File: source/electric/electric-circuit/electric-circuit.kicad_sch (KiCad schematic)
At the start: 7 parts

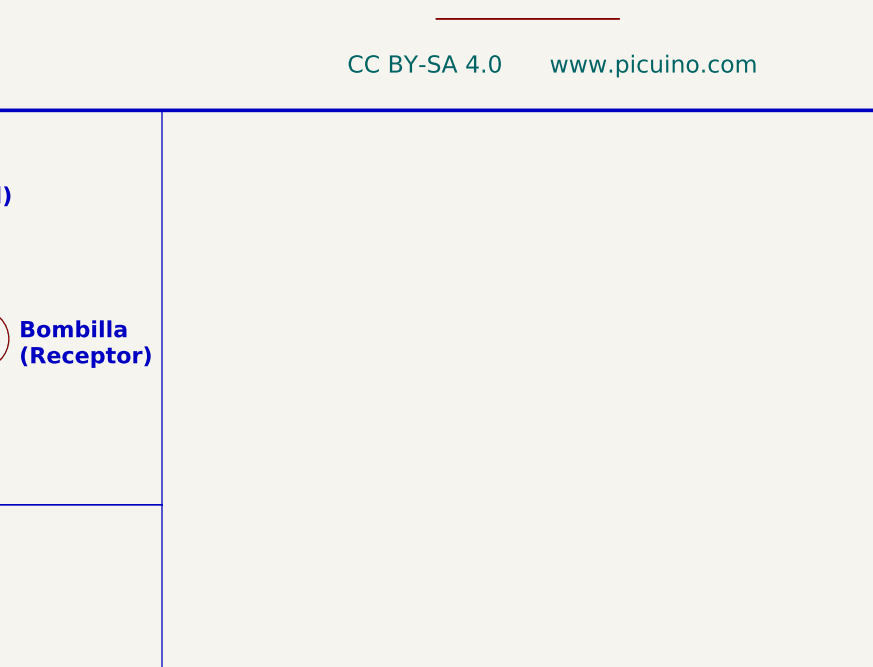
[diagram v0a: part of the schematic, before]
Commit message: 02/09/2024 Update
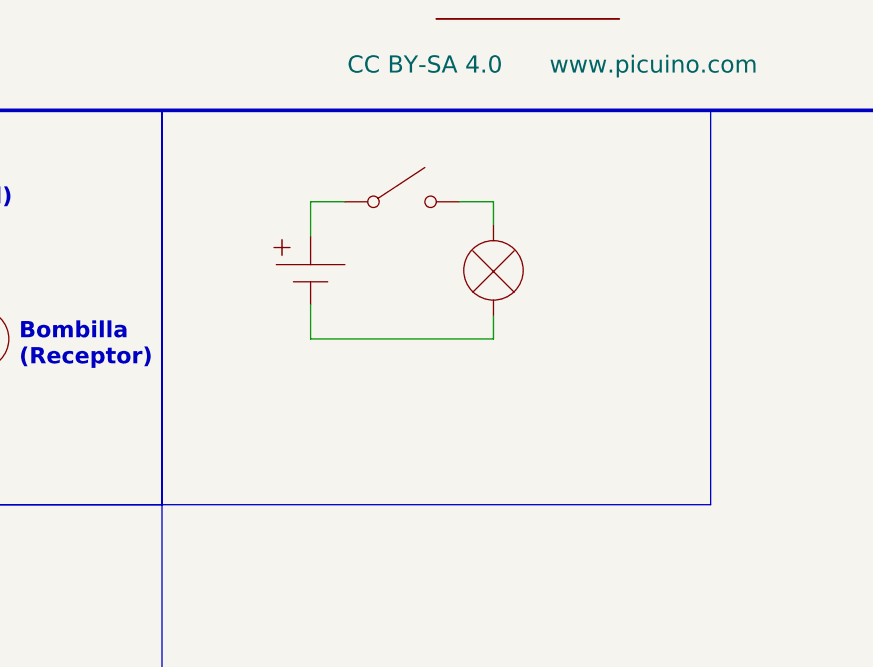
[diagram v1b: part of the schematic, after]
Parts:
- added L2: lampara, symbol simbolos-electricos:lampara
- added S2: interruptor, symbol simbolos-electricos:interruptor
- added V2: Pila, symbol simbolos-electricos:Pila
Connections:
- net at S1.: now also V1.; no longer L1.
- net at V1.: now also L1.; no longer S1.
- net at S3.: now also L3.; no longer V3.
- net at L3.: now also V3.; no longer S3.
- new net: L1., S1.
- new net: S2., V2.
- new net: L2., S2.
- new net: L2., V2.
- new net: S3., V3.
